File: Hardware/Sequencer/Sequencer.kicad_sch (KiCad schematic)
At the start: 10 parts, among them J101 AudioJack2

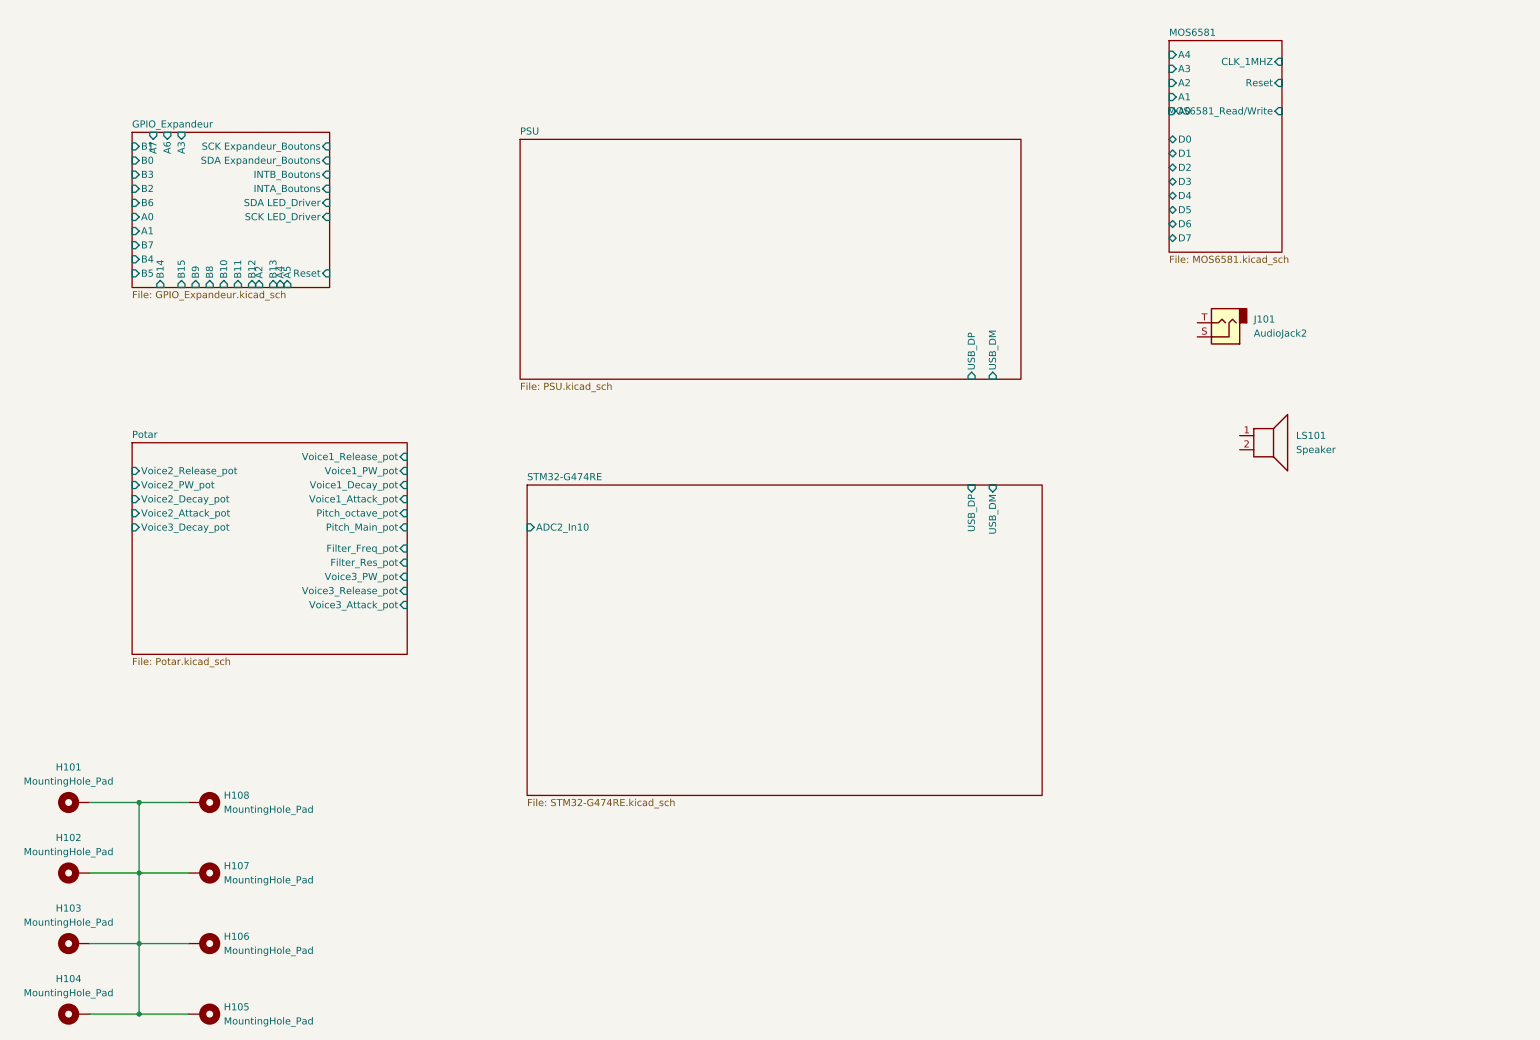
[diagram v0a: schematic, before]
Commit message: pcb
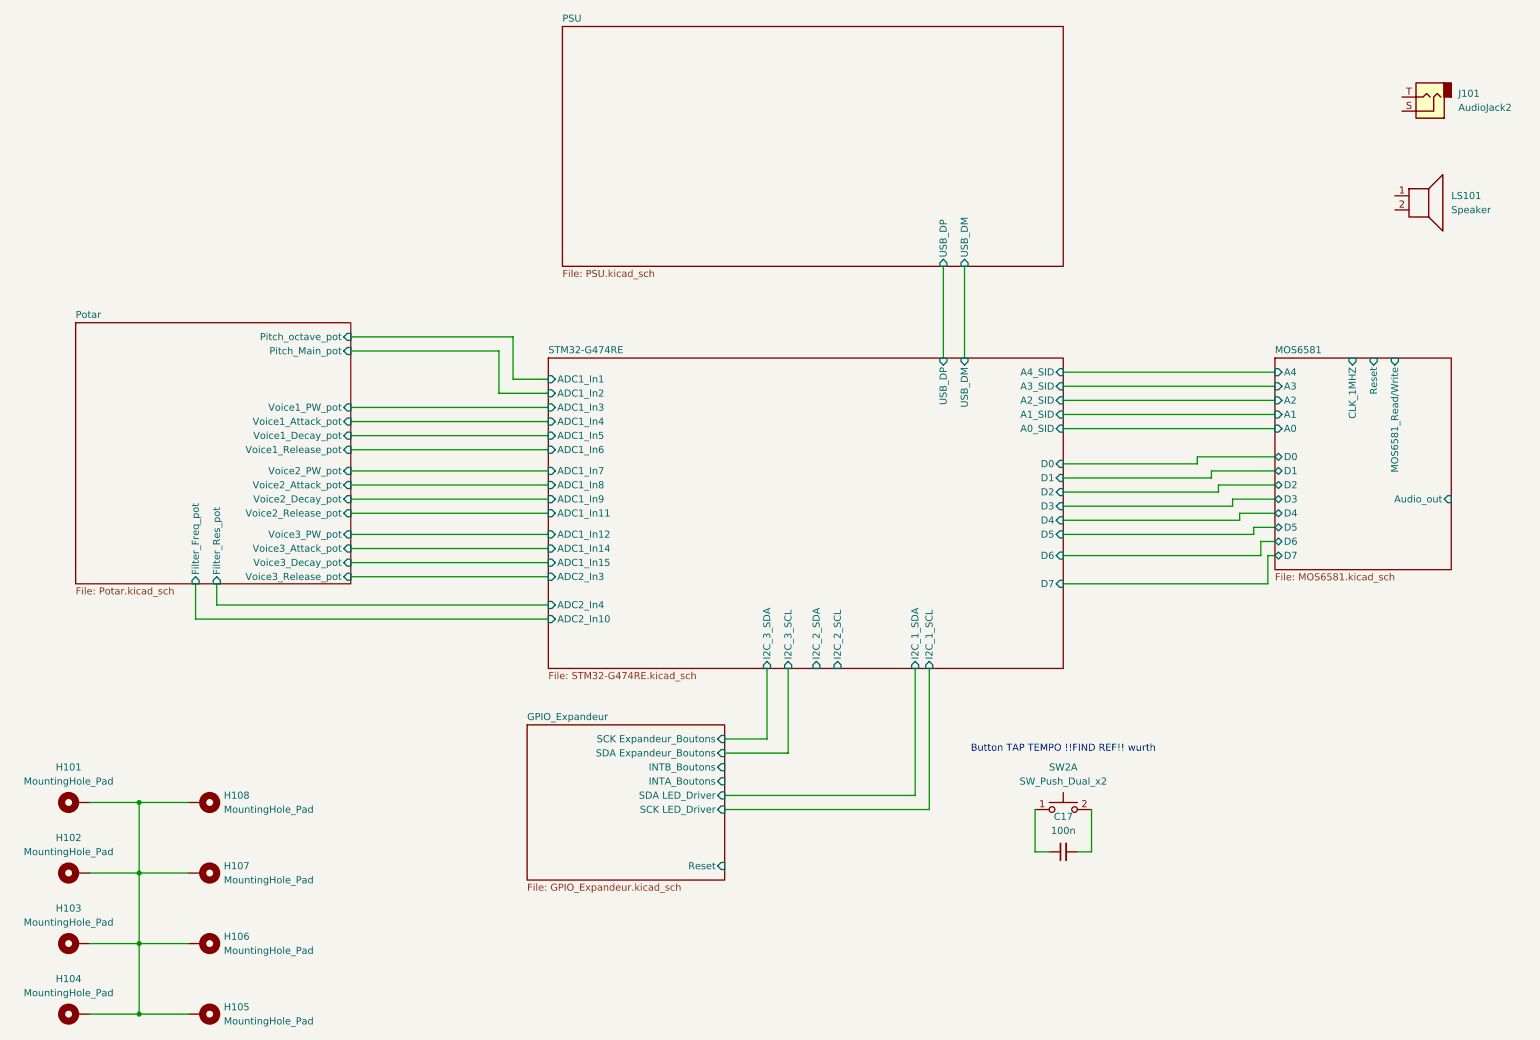
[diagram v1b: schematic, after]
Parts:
- added C17: 100n, Capacitor_SMD:C_0402_1005Metric, symbol Device:C_Small
- added SW2: SW_Push_Dual_x2, symbol Switch:SW_Push_Dual_x2
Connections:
- new net: C17.1, SW2.1 (C)
- new net: C17.2, SW2.2 (D)
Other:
- sheet GPIO_Expandeur ports: added none; removed A0, A1, A2, A3, A4, A5, A6, A7, B0, B1, B10, B11, B12, B13, B14, B15, B2, B3, B4, B5, B6, B7, B8, B9
- sheet MOS6581 ports: added Audio_out; removed none
- sheet STM32-G474RE ports: added A0_SID, A1_SID, A2_SID, A3_SID, A4_SID, ADC1_In1, ADC1_In11, ADC1_In12, ADC1_In14, ADC1_In15, ADC1_In2, ADC1_In3, ADC1_In4, ADC1_In5, ADC1_In6, ADC1_In7, ADC1_In8, ADC1_In9, ADC2_In3, ADC2_In4, D0, D1, D2, D3, D4, D5, D6, D7, I2C_1_SCL, I2C_1_SDA, I2C_2_SCL, I2C_2_SDA, I2C_3_SCL, I2C_3_SDA; removed none
- note added: "Button TAP TEMPO !!FIND REF!! wurth"
- moved on the sheet: J101, LS101
